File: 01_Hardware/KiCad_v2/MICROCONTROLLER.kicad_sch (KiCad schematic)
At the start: 33 parts, among them Q500 IRLML2402TRPBF, U500 DS3231M, U501 ESP32-WROOM-32E-N4, U502 AT24CS01-SSHM

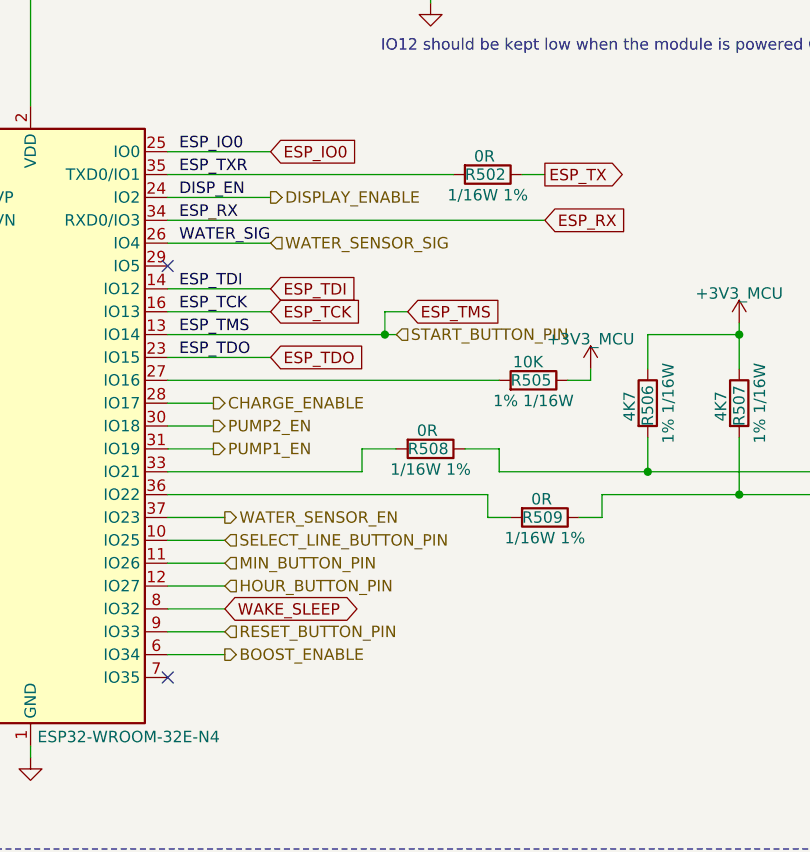
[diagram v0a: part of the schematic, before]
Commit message: Hardware for manufacturing v0.2
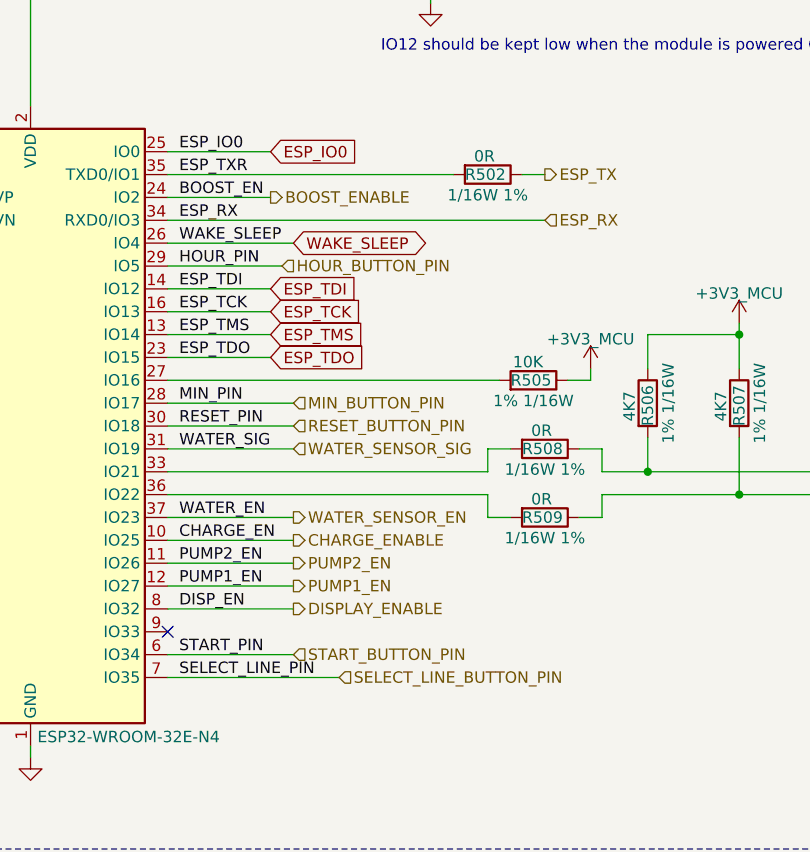
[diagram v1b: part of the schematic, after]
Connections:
- net BOOST_ENABLE: now also U501.24 (IO2); no longer U501.6 (IO34)
- net CHARGE_ENABLE: now also U501.10 (IO25); no longer U501.28 (IO17)
- net DISPLAY_ENABLE: now also U501.8 (IO32); no longer U501.24 (IO2)
- net HOUR_BUTTON_PIN: now also U501.29 (IO5); no longer U501.12 (IO27)
- net MIN_BUTTON_PIN: now also U501.28 (IO17); no longer U501.11 (IO26)
- net PUMP1_EN: now also U501.12 (IO27); no longer U501.31 (IO19)
- net PUMP2_EN: now also U501.11 (IO26); no longer U501.30 (IO18)
- net RESET_BUTTON_PIN: now also U501.30 (IO18); no longer U501.9 (IO33)
- net SELECT_LINE_BUTTON_PIN: now also U501.7 (IO35); no longer U501.10 (IO25)
- net WAKE_SLEEP: now also U501.26 (IO4); no longer U501.8 (IO32)
- net WATER_SENSOR_SIG: now also U501.31 (IO19); no longer U501.26 (IO4)
- new net START_BUTTON_PIN: U501.6 (IO34)
- no-connect marks 5 -> 4
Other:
- moved on the sheet: R508
